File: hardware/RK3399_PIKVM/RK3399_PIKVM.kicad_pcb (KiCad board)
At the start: 6 copper layers, 8 parts

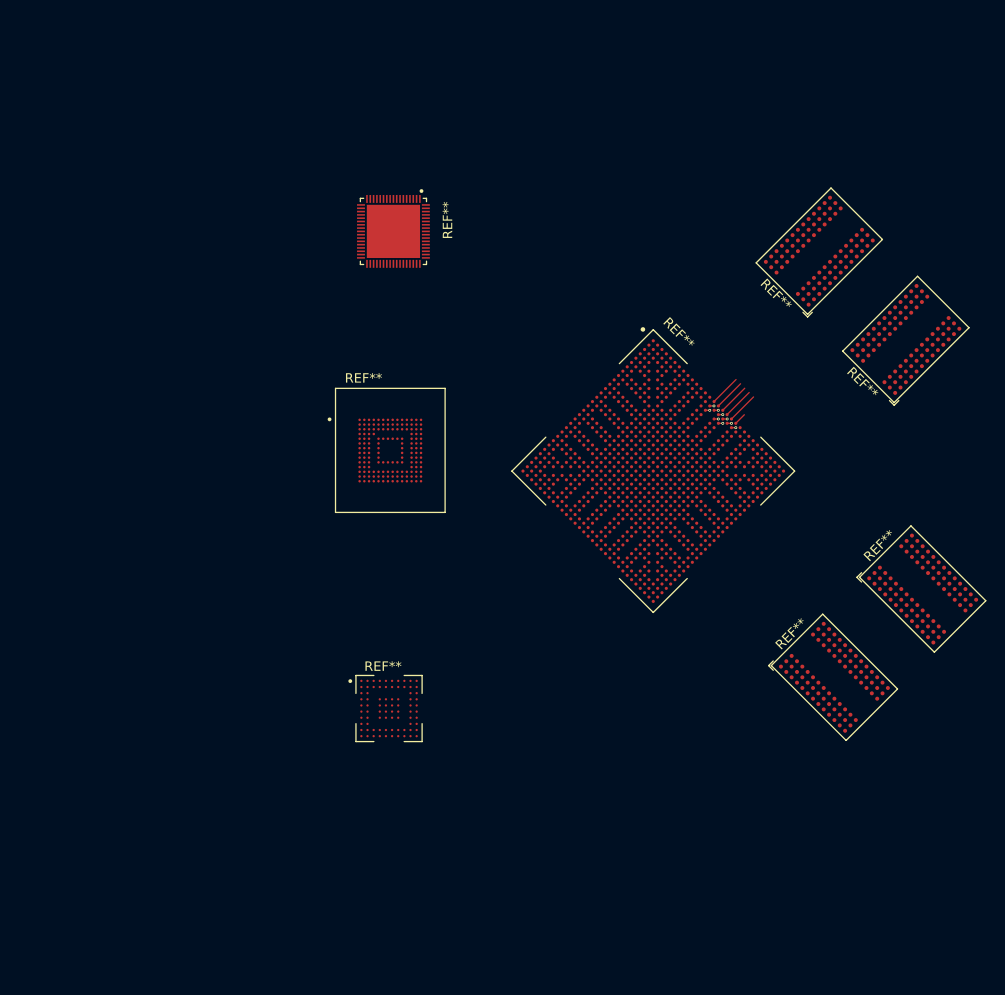
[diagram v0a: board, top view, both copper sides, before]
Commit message: Made a testing design.
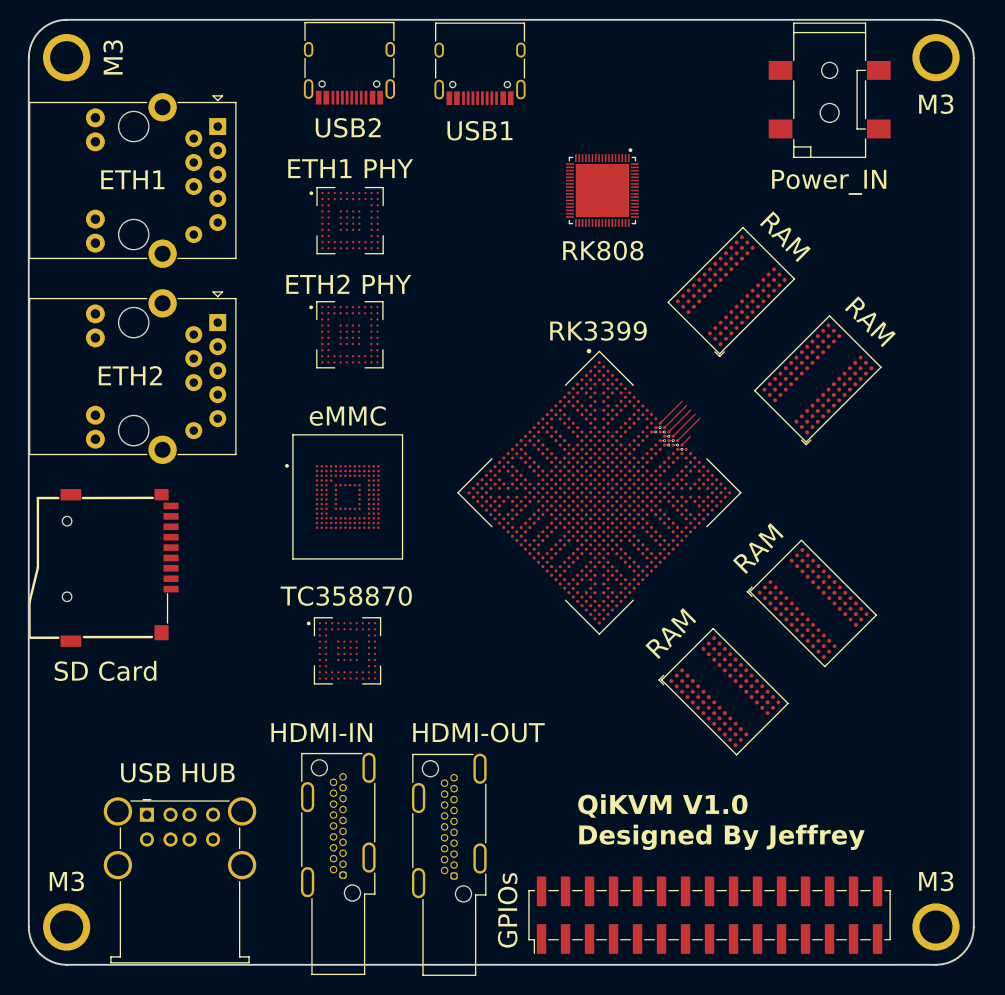
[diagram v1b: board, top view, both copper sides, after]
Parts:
- added ETH1: RJ45_Abracon_ARJP11A-MA_Horizontal, Connector_RJ:RJ45_Abracon_ARJP11A-MA_Horizontal, F.Cu at (90.0, 61.3)
- added ETH1 PHY: BGA80C65P10X10_700X700X100N, zgoolib:TC358870XBG, F.Cu at (104.0, 71.3)
- added ETH2: RJ45_Abracon_ARJP11A-MA_Horizontal, Connector_RJ:RJ45_Abracon_ARJP11A-MA_Horizontal, F.Cu at (90.0, 82.0)
- added ETH2 PHY: BGA80C65P10X10_700X700X100N, zgoolib:TC358870XBG, F.Cu at (104.0, 83.3)
- added GPIOs: PinHeader_2x15_P2.54mm_Vertical_SMD, Connector_PinHeader_2.54mm:PinHeader_2x15_P2.54mm_Vertical_SMD, F.Cu at (142.0, 144.8)
- added HDMI-IN: HDMI_A_Kycon_KDMIX-SL1-NS-WS-B15_VerticalRightAngle, Connector_HDMI:HDMI_A_Kycon_KDMIX-SL1-NS-WS-B15_VerticalRightAngle, F.Cu at (103.2, 140.5)
- added HDMI-OUT: HDMI_A_Kycon_KDMIX-SL1-NS-WS-B15_VerticalRightAngle, Connector_HDMI:HDMI_A_Kycon_KDMIX-SL1-NS-WS-B15_VerticalRightAngle, F.Cu at (115.0, 140.6)
- added M3: M3_Whole, zgoolib:M3_Whole, F.Cu at (74.0, 54.0)
- added M3: M3_Whole, zgoolib:M3_Whole, F.Cu at (166.0, 146.0)
- added M3: M3_Whole, zgoolib:M3_Whole, F.Cu at (166.0, 54.0)
- added M3: M3_Whole, zgoolib:M3_Whole, F.Cu at (74.0, 146.0)
- added Power_IN: DC-05_SMD, zgoolib:DC-05_SMD, F.Cu at (154.7, 59.5)
- added SD Card: TF-SMD_TF-02, zgoolib:TF-SMD_TF-02, F.Cu at (79.7, 108.0)
- added USB HUB: USB_A_Wuerth_61400826021_Horizontal_Stacked, Connector_USB:USB_A_Wuerth_61400826021_Horizontal_Stacked, F.Cu at (82.5, 134.1)
- added USB1: USB_C_Receptacle_HRO_TYPE-C-31-M-12, Connector_USB:USB_C_Receptacle_HRO_TYPE-C-31-M-12, F.Cu at (117.7, 54.3)
- added USB2: USB_C_Receptacle_HRO_TYPE-C-31-M-12, Connector_USB:USB_C_Receptacle_HRO_TYPE-C-31-M-12, F.Cu at (103.9, 54.2)
- moved RK808 22.5 mm to (130.7, 68.1)
- moved RAM 11.7 mm to (153.0, 111.8)
- moved RAM 11.7 mm to (143.7, 121.1)
- moved RAM 10.2 mm to (153.5, 88.0)
- moved RAM 10.2 mm to (144.3, 78.7)
- moved TC358870 7.52 mm to (103.7, 116.8)
- moved eMMC 6.67 mm to (103.7, 100.5)
- moved RK3399 6.15 mm to (130.4, 100.0)
- renumbered REF** to RAM, REF** to RK3399, REF** to RK808, REF** to TC358870, REF** to eMMC
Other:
- board outline added: 100 x 100 mm
- board text added: "QiKVM V1.0 Designed By Jeffrey"
